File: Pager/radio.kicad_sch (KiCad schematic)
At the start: 26 parts, among them U4 CC1101RGPR, Y1 26 MHz

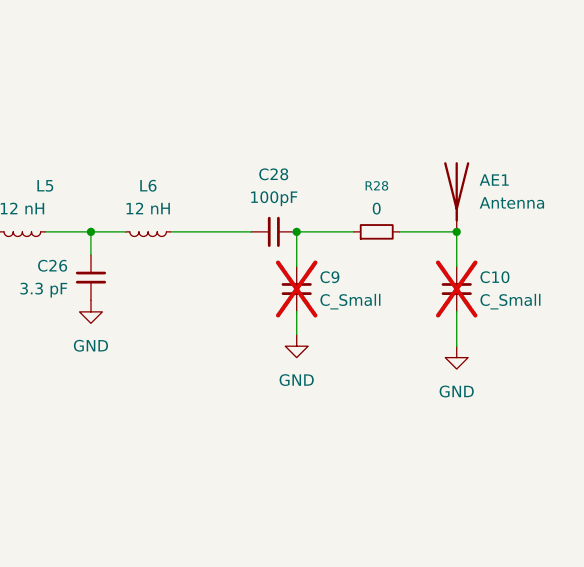
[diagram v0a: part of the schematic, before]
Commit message: updated
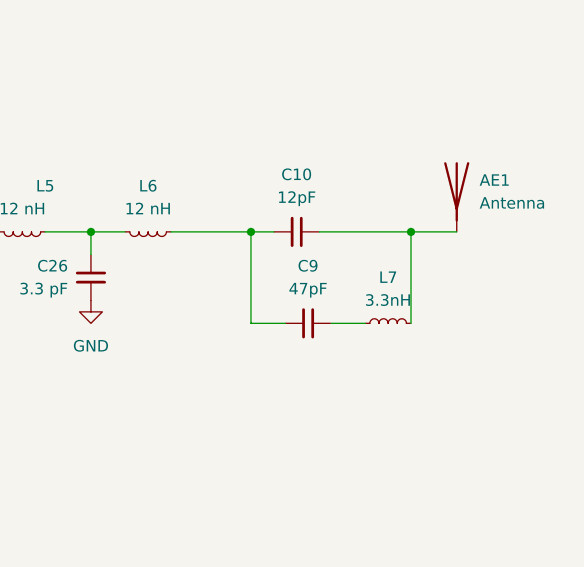
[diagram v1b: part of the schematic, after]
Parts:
- removed C28: 100pF, Capacitor_SMD:C_0402_1005Metric, symbol Device:C_Small
- removed R28: 0, Resistor_SMD:R_0402_1005Metric, symbol Device:R_Small
- added L7: 3.3nH, symbol Device:L_Small
- C10: value C_Small -> 12pF; footprint Capacitor_SMD:C_0402_1005Metric -> (none); now fitted
- C15, C16, C17, C18, C19, C20, C21, C22, C23, C24, C25, C26: footprint Capacitor_SMD:C_0402_1005Metric -> Capacitor_SMD:C_0805_2012Metric_Pad1.18x1.45mm_HandSolder
- C9: value C_Small -> 47pF; footprint Capacitor_SMD:C_0402_1005Metric -> (none); now fitted
- L1, L2, L3, L4, L5, L6: footprint Inductor_SMD:L_0402_1005Metric -> Inductor_SMD:L_0805_2012Metric_Pad1.05x1.20mm_HandSolder
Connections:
- net GND: no longer C10.2, C9.2
- net at L6.1: now also C10.1, C9.1
- net at AE1.1 (A): now also C10.2, L7.2; no longer C10.1
- new net: C9.2, L7.1

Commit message: layout
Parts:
- C10, C9: footprint (none) -> Capacitor_SMD:C_0805_2012Metric_Pad1.18x1.45mm_HandSolder
- L7: footprint (none) -> Inductor_SMD:L_0805_2012Metric_Pad1.05x1.20mm_HandSolder
- R13: footprint Resistor_SMD:R_0402_1005Metric -> Resistor_SMD:R_0805_2012Metric_Pad1.20x1.40mm_HandSolder
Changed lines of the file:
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@@
 			)
 		)
-		(property "Footprint" ""
+		(property "Footprint" "Inductor_SMD:L_0805_2012Metric_Pad1.05x1.20mm_HandSolder"
 			(at 207.01 102.87 0)
 			(hide yes)
@@
 			)
 		)
-		(property "Footprint" ""
+		(property "Footprint" "Capacitor_SMD:C_0805_2012Metric_Pad1.18x1.45mm_HandSolder"
 			(at 196.85 92.71 0)
 			(hide yes)
@@
 			)
 		)
-		(property "Footprint" ""
+		(property "Footprint" "Capacitor_SMD:C_0805_2012Metric_Pad1.18x1.45mm_HandSolder"
 			(at 198.12 102.87 0)
 			(hide yes)
@@
 			)
 		)
-		(property "Footprint" "Resistor_SMD:R_0402_1005Metric"
+		(property "Footprint" "Resistor_SMD:R_0805_2012Metric_Pad1.20x1.40mm_HandSolder"
 			(at 96.52 60.96 0)
 			(hide yes)
